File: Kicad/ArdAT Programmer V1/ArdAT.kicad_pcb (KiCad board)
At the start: 2 copper layers, 75 x 75 mm, 24 parts, among them J1 Audio-Jack-2, J2 Conn_01x06, U1 LM317A-SMD

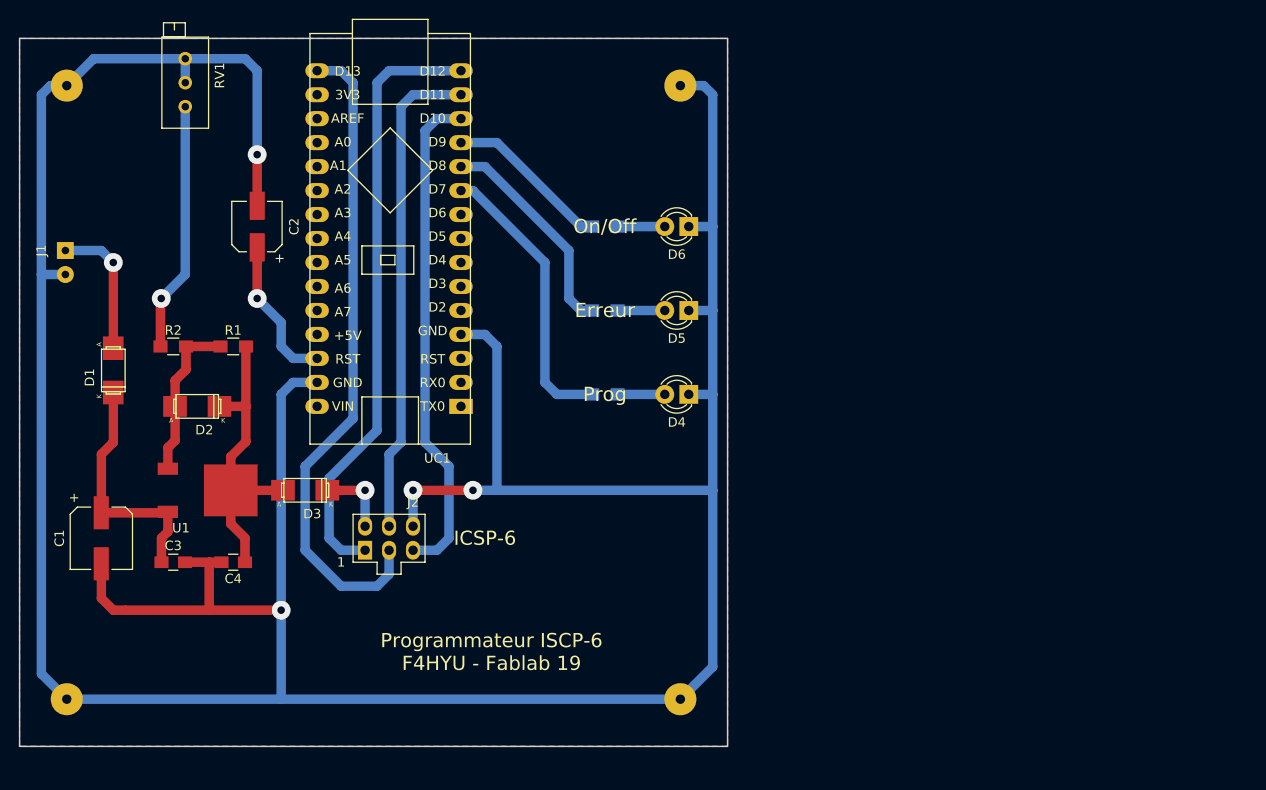
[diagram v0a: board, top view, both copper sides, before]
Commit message: Update
Update
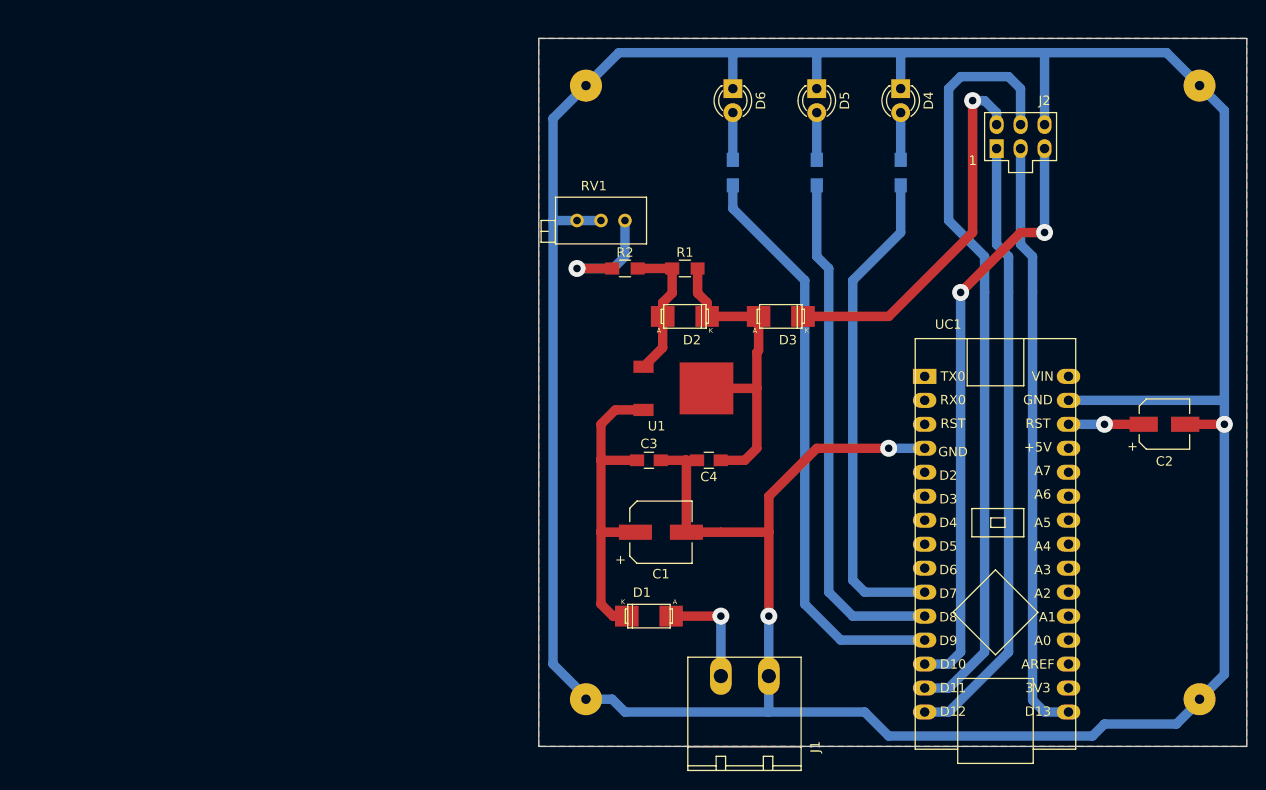
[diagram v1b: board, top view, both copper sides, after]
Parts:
- J1: footprint alex-library:Connect-2pin -> alex-library:Connecteur-Embase-Debrochable-2_Voies
- moved H1 136.5 mm to (190.0, 60.0)
- moved C2 98.4 mm to (186.3, 95.9), turned to 0 degrees
- moved H3 85.1 mm to (125.0, 125.0)
- moved H4 85.1 mm to (190.0, 125.0)
- moved J1 82.8 mm to (139.3, 122.5), turned to 90 degrees
- moved J2 79.3 mm to (168.5, 66.7)
- moved H2 65.8 mm to (125.0, 60.0)
- moved D1 62.4 mm to (131.7, 116.2), turned to 0 degrees
- moved C1 59.3 mm to (132.9, 107.3), turned to 0 degrees
- moved D3 53.7 mm to (145.6, 84.5)
- moved D2 52.5 mm to (135.5, 84.5)
- moved C4 51.5 mm to (138.0, 99.7)
- moved U1 51.5 mm to (135.5, 92.1)
- moved C3 51.5 mm to (131.7, 99.7)
- moved UC1 49.2 mm to (160.9, 90.8), turned to 0 degrees
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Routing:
- net Net-(R5-Pad2): track 17.6 -> 61.8 mm
- net VCC: track 7.81 -> 40.0 mm
- net Net-(R4-Pad2): track 23.2 -> 54.8 mm
- net MOSI: track 51.9 -> 81.7 mm
- net Net-(R3-Pad2): track 30.3 -> 52.1 mm
- net Net-(R2-Pad1): track 26.5 -> 13.1 mm
- net RESET: track 52.9 -> 62.8 mm, vias 0 -> 2
- net Net-(C1-Pad1): track 26.0 -> 34.9 mm
- net Net-(C2-Pad1): track 15.9 -> 7.96 mm
- net SCK: track 69.5 -> 63.3 mm
- net Net-(D1-Pad2): track 14.7 -> 11.6 mm
- net GND: track 375.3 -> 377.9 mm, vias 4 -> 3
- net Net-(D2-Pad2): track 17.4 -> 15.3 mm
- net Net-(C4-Pad1): track 32.6 -> 34.7 mm
- net MISO: track 64.1 -> 65.4 mm
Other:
- rule pad_to_mask_clearance: 0.2 -> 0
- board text added: "2.7V"
- board text added: "3.3V"
- board text added: "5-12V C.C"
- board text added: "Adj 3.3V"
- board text added: "F4HYU"
- board text added: "Fablab19"
- board text added: "GND"
- board text added: "Programmateur Universel"
- board text added: "USB"
- board text removed: "Programmateur ISCP-6 F4HYU - Fablab 19"
